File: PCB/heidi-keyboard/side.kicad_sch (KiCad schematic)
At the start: 53 parts, among them SW1 SW_Push, SW11 SW_Push, SW13 SW_Push, SW15 SW_Push, SW17 SW_Push, SW19 SW_Push, SW21 SW_Push, SW23 SW_Push, SW25 SW_Push, SW27 SW_Push, SW29 SW_Push, SW3 SW_Push, SW31 SW_Push, SW33 SW_Push, SW35 SW_Push, SW37 SW_Push, SW39 SW_Push, SW49 SW_Push, SW5 SW_Push, SW51 SW_Push, SW53 SW_Push, SW55 SW_Push, SW57 SW_Push, SW7 SW_Push, SW9 SW_Push, U1 XIAO-nRF52840-SMD

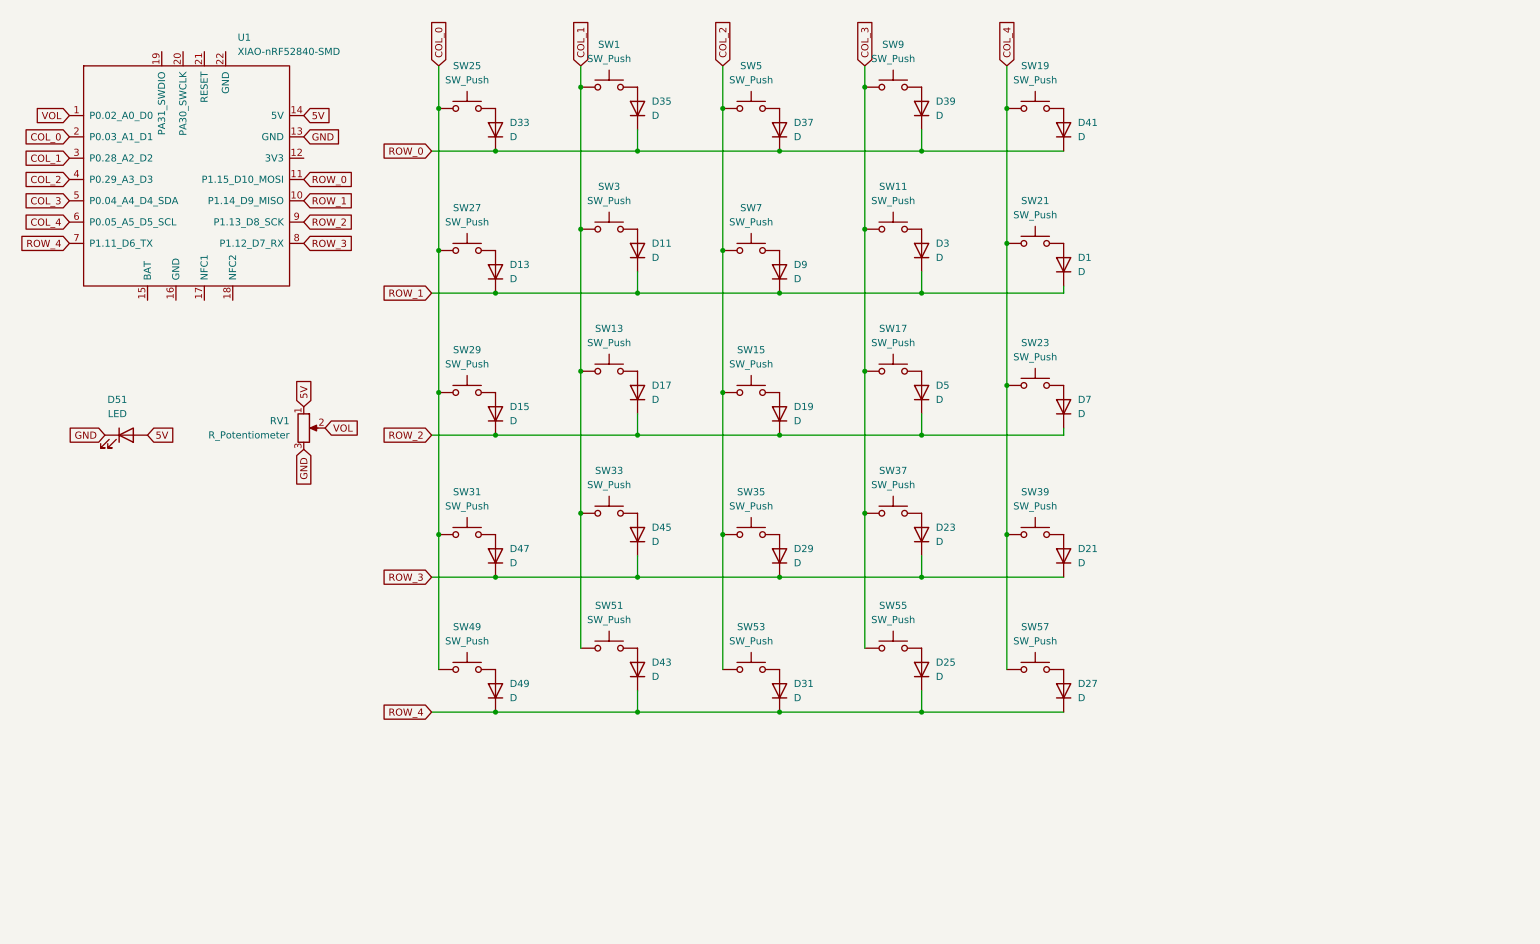
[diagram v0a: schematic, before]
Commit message: aaaaaaaaaa
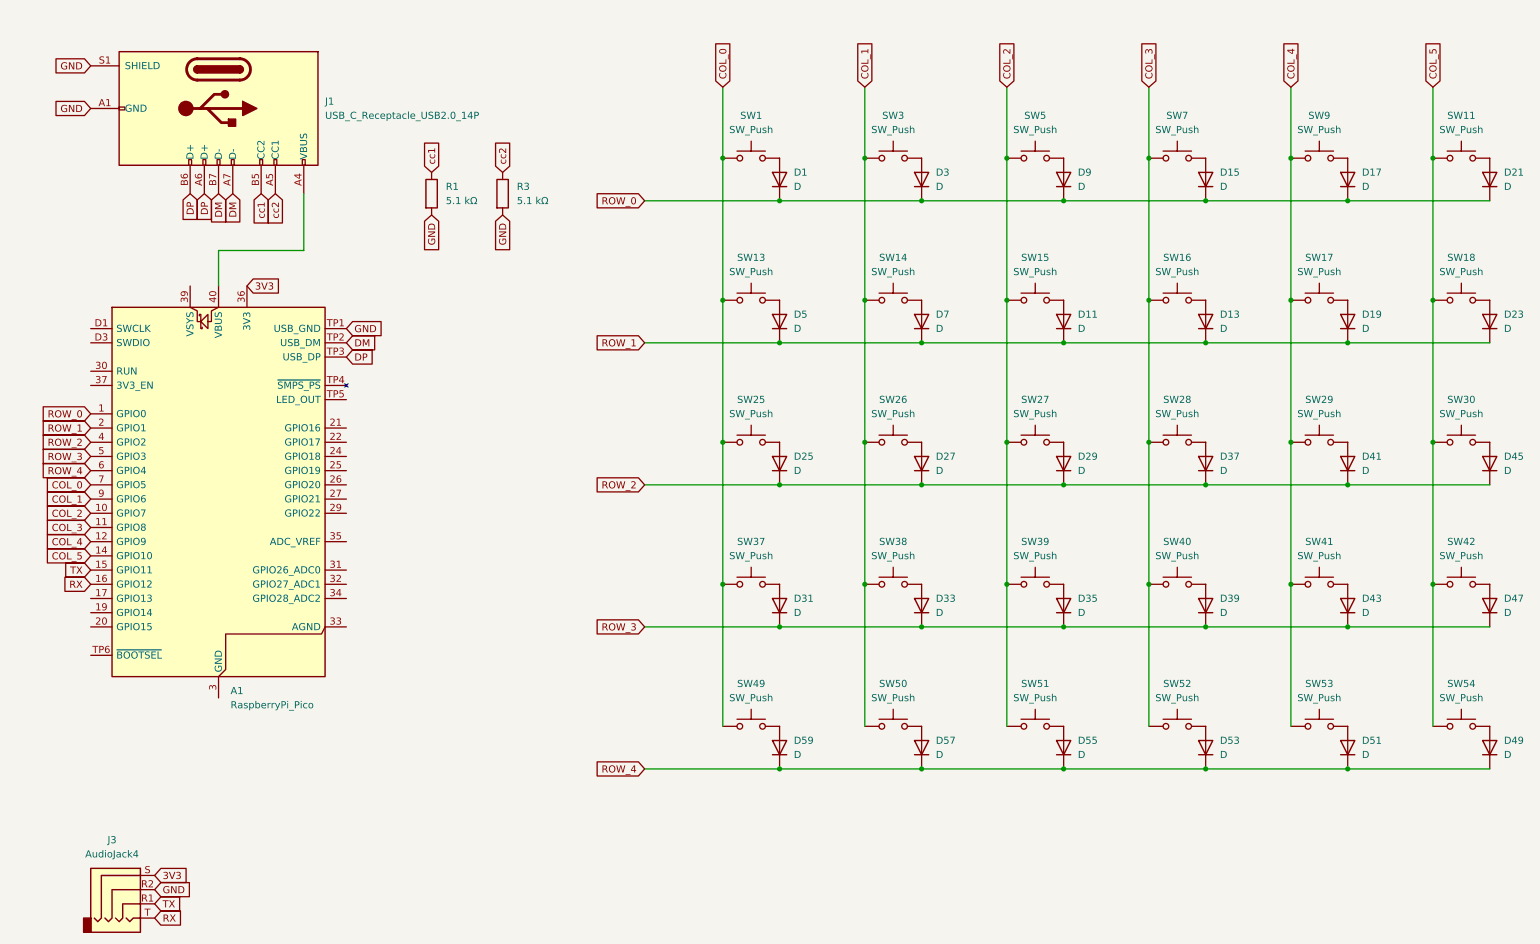
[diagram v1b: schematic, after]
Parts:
- removed D51: LED, symbol Device:LED
- removed RV1: R_Potentiometer, symbol Device:R_Potentiometer
- removed SW19, SW21, SW23, SW31, SW33, SW35, SW55, SW57: SW_Push, symbol Switch:SW_Push
- removed U1: XIAO-nRF52840-SMD, symbol OPL:XIAO-nRF52840-SMD
- added A1: RaspberryPi_Pico, Module:RaspberryPi_Pico_SMD, symbol MCU_Module:RaspberryPi_Pico_Extensive
- added D51, D53, D55, D57, D59: D, symbol Device:D
- added J1: USB_C_Receptacle_USB2.0_14P, symbol Connector:USB_C_Receptacle_USB2.0_14P
- added J3: AudioJack4, symbol Connector_Audio:AudioJack4
- added R1, R3: 5.1 kΩ, symbol Device:R
- added SW14, SW16, SW18, SW26, SW28, SW30, SW38, SW40, SW41, SW42, SW50, SW52, SW54: SW_Push, symbol Switch:SW_Push
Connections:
- net COL_0: now also SW1.1, SW13.1, SW37.1, A1.7 (GPIO5); no longer SW27.1, SW29.1
- net COL_1: now also A1.9 (GPIO6), SW14.1, SW26.1, SW38.1, SW50.1; no longer SW1.1, SW13.1, SW51.1
- net COL_2: now also SW27.1, SW39.1, SW51.1, A1.10 (GPIO7); no longer SW53.1, SW7.1
- net COL_3: now also SW7.1, A1.11 (GPIO8), SW16.1, SW28.1, SW40.1, SW52.1; no longer SW11.1, SW17.1, SW37.1, SW9.1
- net COL_4: now also SW17.1, SW29.1, SW53.1, SW9.1, A1.12 (GPIO9), SW41.1; no longer SW39.1
- net GND: now also A1.TP1 (USB_GND), J1.A1 (GND), J1.A12 (GND), J1.B1 (GND), J1.B12 (GND), J1.S1 (SHIELD), J3.R2, R1.2, R3.2
- net ROW_0: now also D1.1 (K), D15.1 (K), D17.1 (K), D21.1 (K), D3.1 (K), D9.1 (K), A1.1 (GPIO0); no longer D33.1 (K), D35.1 (K), D37.1 (K), D39.1 (K), D41.1 (K)
- net ROW_1: now also D19.1 (K), D23.1 (K), D5.1 (K), D7.1 (K), A1.2 (GPIO1); no longer D1.1 (K), D3.1 (K), D9.1 (K)
- net ROW_2: now also D25.1 (K), D27.1 (K), D29.1 (K), D37.1 (K), D41.1 (K), D45.1 (K), A1.4 (GPIO2); no longer D15.1 (K), D17.1 (K), D19.1 (K), D5.1 (K), D7.1 (K)
- net ROW_3: now also D31.1 (K), D33.1 (K), D35.1 (K), D39.1 (K), D43.1 (K), A1.5 (GPIO3); no longer D21.1 (K), D23.1 (K), D29.1 (K), D45.1 (K)
- net ROW_4: now also A1.6 (GPIO4), D51.1 (K), D53.1 (K), D55.1 (K), D57.1 (K), D59.1 (K); no longer D25.1 (K), D27.1 (K), D31.1 (K), D43.1 (K)
- net at SW7.2: now also D15.2 (A); no longer D9.2 (A)
- net at D27.2 (A): now also SW26.2
- net at SW17.2: now also D19.2 (A); no longer D5.2 (A)
- net at D21.2 (A): now also SW11.2; no longer SW39.2
- net at D31.2 (A): now also SW37.2; no longer SW53.2
- net at D33.2 (A): now also SW38.2; no longer SW25.2
- net at D11.2 (A): now also SW15.2; no longer SW3.2
- net at SW13.2: now also D5.2 (A); no longer D17.2 (A)
- net at SW29.2: now also D41.2 (A); no longer D15.2 (A)
- net at D29.2 (A): now also SW27.2
- net at D25.2 (A): now also SW25.2
- net at SW5.2: now also D9.2 (A); no longer D37.2 (A)
- net at D47.2 (A): now also SW42.2
- net at D23.2 (A): now also SW18.2; no longer SW37.2
- net at SW49.2: now also D59.2 (A); no longer D49.2 (A)
- net at D43.2 (A): now also SW41.2; no longer SW51.2
- net at D3.2 (A): now also SW3.2; no longer SW11.2
- net at D39.2 (A): now also SW40.2; no longer SW9.2
- net at D1.2 (A): now also SW1.2
- net at D7.2 (A): now also SW14.2
- net at D35.2 (A): now also SW39.2; no longer SW1.2
- net at D45.2 (A): now also SW30.2
- net at D13.2 (A): now also SW16.2; no longer SW27.2
- new net: D49.2 (A), SW54.2
- new net: D53.2 (A), SW52.2
- new net: A1.13 (GND), A1.18 (GND), A1.23 (GND), A1.28 (GND), A1.3 (GND), A1.38 (GND), A1.8 (GND), A1.D2 (GND)
- new net: A1.40 (VBUS), J1.A4 (VBUS), J1.A9 (VBUS), J1.B4 (VBUS), J1.B9 (VBUS)
- new net: D57.2 (A), SW50.2
- new net: D37.2 (A), SW28.2
- new net: D55.2 (A), SW51.2
- new net: D17.2 (A), SW9.2
- new net: D51.2 (A), SW53.2
- new net 3V3: A1.36 (3V3), J3.S
- new net COL_5: A1.14 (GPIO10), SW11.1, SW18.1, SW30.1, SW42.1, SW54.1
- new net DM: A1.TP2 (USB_DM), J1.A7 (D-), J1.B7 (D-)
- new net DP: A1.TP3 (USB_DP), J1.A6 (D+), J1.B6 (D+)
- new net RX: A1.16 (GPIO12), J3.T
- new net TX: A1.15 (GPIO11), J3.R1
- new net cc1: J1.B5 (CC2), R1.1
- new net cc2: J1.A5 (CC1), R3.1
